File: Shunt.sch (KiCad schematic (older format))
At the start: 1 part

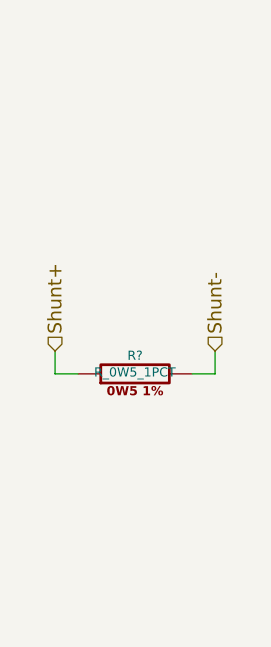
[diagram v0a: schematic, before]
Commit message: working on revamp of power supply.
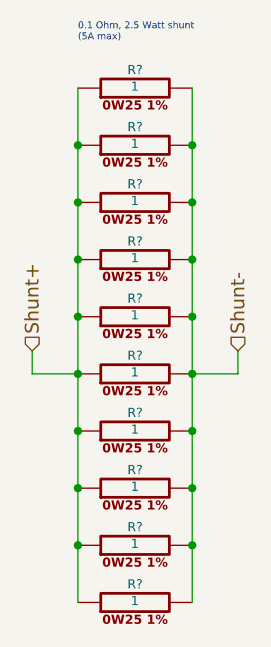
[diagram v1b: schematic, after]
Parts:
- removed R?: R_0W5_1PCT, ~, symbol R_0W5_1PCT
- added R? (x10): 1, ~, symbol R_0W25_1PCT
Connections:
- net Shunt+: now also R?.1, R?.1, R?.1, R?.1, R?.1, R?.1, R?.1, R?.1, R?.1, R?.1
- net Shunt-: now also R?.2, R?.2, R?.2, R?.2, R?.2, R?.2, R?.2, R?.2, R?.2, R?.2
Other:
- note added: "0.1 Ohm, 2.5 Watt shunt\n(5A max)"
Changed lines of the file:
@@
 EESchema Schematic File Version 2
+LIBS:references_PL
+LIBS:OpAmpPassXsistorBenchSupply-cache
 LIBS:opamps_PL
+LIBS:opto_PL
+LIBS:regulators_PL
+LIBS:relays_PL
+LIBS:resistors_PL
+LIBS:switches_PL
 LIBS:transistors_PL
+LIBS:analog_ICs_PL
+LIBS:capacitors_PL
+LIBS:connectors_PL
 LIBS:diodes_PL
-LIBS:resistors_PL
-LIBS:capacitors_PL
-LIBS:regulators_PL
-LIBS:connectors_PL
+LIBS:displays_PL
+LIBS:LEDs_PL
+LIBS:microcontrollers_PL
+LIBS:mounting_holes_PL
 LIBS:power
 LIBS:device
@@
 $Descr A4 11693 8268
 encoding utf-8
-Sheet 8 9
+Sheet 4 2
 Title ""
 Date "4 jul 2014"
@@
 Comment4 ""
 $EndDescr
-$Comp
-L R_0W5_1PCT R?
-U 1 1 53383531
+Wire Wire Line
+	5150 3800 5150 3900
+Wire Wire Line
+	6050 3800 6050 3900
+Wire Wire Line
+	5150 3900 5350 3900
+Wire Wire Line
+	6050 3900 5850 3900
+Text HLabel 5150 3800 1    60   Input ~ 0
+Shunt+
+Text HLabel 6050 3800 1    60   Input ~ 0
+Shunt-
+$Comp
+L R_0W25_1PCT R?
+U 1 1 53B6360E
 P 5600 3900
 F 0 "R?" V 5680 3900 40  0000 C CNN
-F 1 "R_0W5_1PCT" V 5607 3901 40  0000 C CNN
+F 1 "1" V 5607 3901 40  0000 C CNN
 F 2 "~" V 5530 3900 30  0000 C CNN
 F 3 "~" H 5600 3900 30  0000 C CNN
@@
 	0    -1   -1   0
 $EndComp
-Wire Wire Line
-	5250 3800 5250 3900
-Wire Wire Line
-	5950 3800 5950 3900
-Wire Wire Line
-	5250 3900 5350 3900
-Wire Wire Line
-	5950 3900 5850 3900
-Text HLabel 5250 3800 1    60   Input ~ 0
-Shunt+
-Text HLabel 5950 3800 1    60   Input ~ 0
-Shunt-
+$Comp
+L R_0W25_1PCT R?
+U 1 1 53B63620
+P 5600 4150
+F 0 "R?" V 5680 4150 40  0000 C CNN
+F 1 "1" V 5607 4151 40  0000 C CNN
+F 2 "~" V 5530 4150 30  0000 C CNN
+F 3 "~" H 5600 4150 30  0000 C CNN
+	1    5600 4150
+	0    -1   -1   0
+$EndComp
+$Comp
+L R_0W25_1PCT R?
+U 1 1 53B63626
+P 5600 4400
+F 0 "R?" V 5680 4400 40  0000 C CNN
+F 1 "1" V 5607 4401 40  0000 C CNN
+F 2 "~" V 5530 4400 30  0000 C CNN
+F 3 "~" H 5600 4400 30  0000 C CNN
+	1    5600 4400
+	0    -1   -1   0
+$EndComp
+$Comp
+L R_0W25_1PCT R?
+U 1 1 53B6362C
+P 5600 3650
+F 0 "R?" V 5680 3650 40  0000 C CNN
+F 1 "1" V 5607 3651 40  0000 C CNN
+F 2 "~" V 5530 3650 30  0000 C CNN
+F 3 "~" H 5600 3650 30  0000 C CNN
+	1    5600 3650
+	0    -1   -1   0
+$EndComp
+$Comp
+L R_0W25_1PCT R?
+U 1 1 53B63632
+P 5600 3400
+F 0 "R?" V 5680 3400 40  0000 C CNN
+F 1 "1" V 5607 3401 40  0000 C CNN
+F 2 "~" V 5530 3400 30  0000 C CNN
+F 3 "~" H 5600 3400 30  0000 C CNN
+	1    5600 3400
+	0    -1   -1   0
+$EndComp
+$Comp
+L R_0W25_1PCT R?
+U 1 1 53B63638
+P 5600 4650
+F 0 "R?" V 5680 4650 40  0000 C CNN
+F 1 "1" V 5607 4651 40  0000 C CNN
+F 2 "~" V 5530 4650 30  0000 C CNN
+F 3 "~" H 5600 4650 30  0000 C CNN
+	1    5600 4650
+	0    -1   -1   0
+$EndComp
+$Comp
+L R_0W25_1PCT R?
+U 1 1 53B6363E
+P 5600 4900
+F 0 "R?" V 5680 4900 40  0000 C CNN
+F 1 "1" V 5607 4901 40  0000 C CNN
+F 2 "~" V 5530 4900 30  0000 C CNN
+F 3 "~" H 5600 4900 30  0000 C CNN
+	1    5600 4900
+	0    -1   -1   0
+$EndComp
+$Comp
+L R_0W25_1PCT R?
+U 1 1 53B63644
+P 5600 3150
+F 0 "R?" V 5680 3150 40  0000 C CNN
+F 1 "1" V 5607 3151 40  0000 C CNN
+F 2 "~" V 5530 3150 30  0000 C CNN
+F 3 "~" H 5600 3150 30  0000 C CNN
+	1    5600 3150
+	0    -1   -1   0
+$EndComp
+$Comp
+L R_0W25_1PCT R?
+U 1 1 53B6364A
+P 5600 2900
+F 0 "R?" V 5680 2900 40  0000 C CNN
+F 1 "1" V 5607 2901 40  0000 C CNN
+F 2 "~" V 5530 2900 30  0000 C CNN
+F 3 "~" H 5600 2900 30  0000 C CNN
+	1    5600 2900
+	0    -1   -1   0
+$EndComp
+$Comp
+L R_0W25_1PCT R?
+U 1 1 53B63650
+P 5600 2650
+F 0 "R?" V 5680 2650 40  0000 C CNN
+F 1 "1" V 5607 2651 40  0000 C CNN
+F 2 "~" V 5530 2650 30  0000 C CNN
+F 3 "~" H 5600 2650 30  0000 C CNN
+	1    5600 2650
+	0    -1   -1   0
+$EndComp
+Wire Wire Line
+	5350 2650 5350 2900
+Wire Wire Line
+	5350 2900 5350 3150
+Wire Wire Line
+	5350 3150 5350 3400
+Wire Wire Line
+	5350 3400 5350 3650
+Wire Wire Line
+	5350 3650 5350 3900
+Wire Wire Line
+	5350 3900 5350 4150
+Wire Wire Line
+	5350 4150 5350 4400
+Wire Wire Line
+	5350 4400 5350 4650
+Wire Wire Line
+	5350 4650 5350 4900
+Connection ~ 5350 2900
+Connection ~ 5350 3150
+Connection ~ 5350 3400
+Connection ~ 5350 3650
+Wire Wire Line
+	5850 2650 5850 2900
+Wire Wire Line
+	5850 2900 5850 3150
+Wire Wire Line
+	5850 3150 5850 3400
+Wire Wire Line
+	5850 3400 5850 3650
+Wire Wire Line
+	5850 3650 5850 3900
+Wire Wire Line
+	5850 3900 5850 4150
+Wire Wire Line
+	5850 4150 5850 4400
+Wire Wire Line
+	5850 4400 5850 4650
+Wire Wire Line
+	5850 4650 5850 4900
+Connection ~ 5850 2900
+Connection ~ 5850 3150
+Connection ~ 5850 3400
+Connection ~ 5850 3650
+Connection ~ 5850 3900
+Connection ~ 5350 3900
+Connection ~ 5850 4150
+Connection ~ 5350 4150
+Connection ~ 5850 4400
+Connection ~ 5350 4400
+Connection ~ 5850 4650
+Connection ~ 5350 4650
+Text Notes 5350 2450 0    30   ~ 0
+0.1 Ohm, 2.5 Watt shunt\n(5A max)
 $EndSCHEMATC
